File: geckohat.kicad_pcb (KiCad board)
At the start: 2 copper layers, 65 x 56 mm, 37 parts, among them J1 CONN_02X20, J2 TEST_1P, U1 EFM32JG1B100F128GM32, U2 LP2985LV, Y1 38.4 MHz, Y2 32kHz

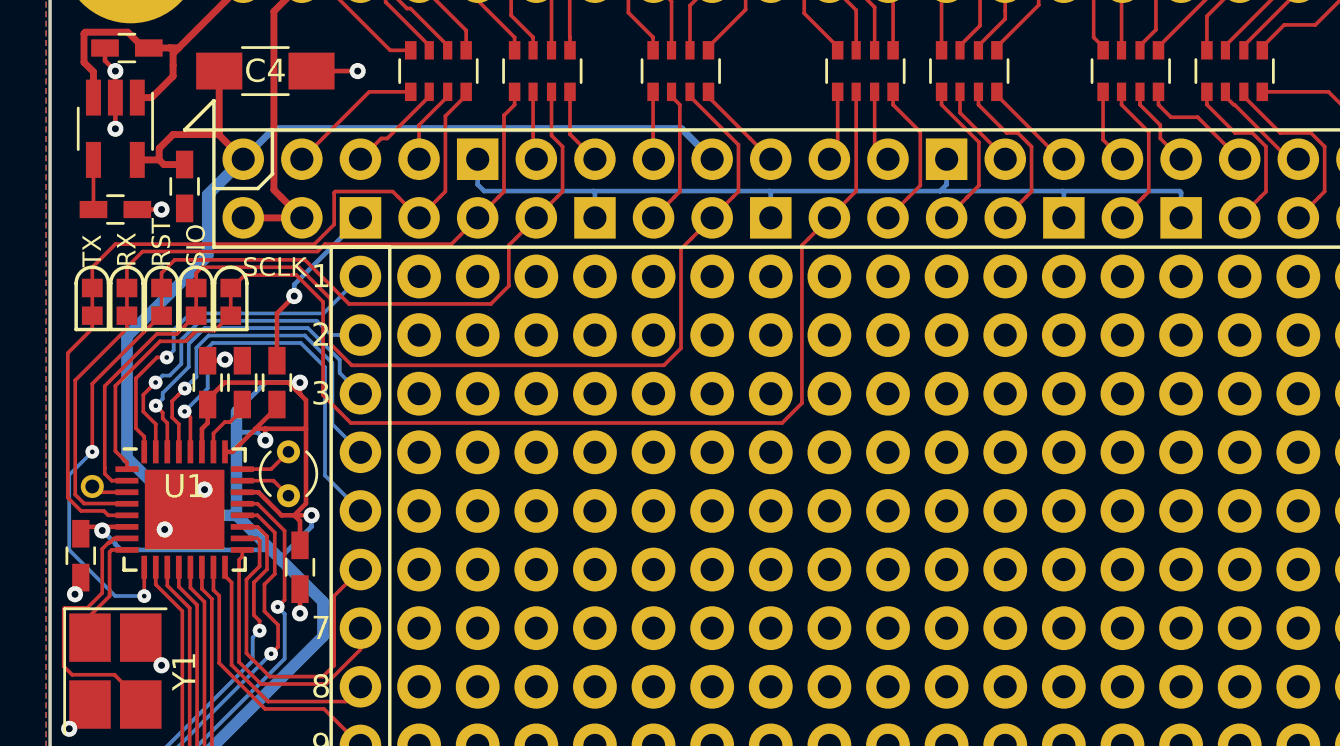
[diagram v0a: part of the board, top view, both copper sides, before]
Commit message: Unknown changes that were lying around
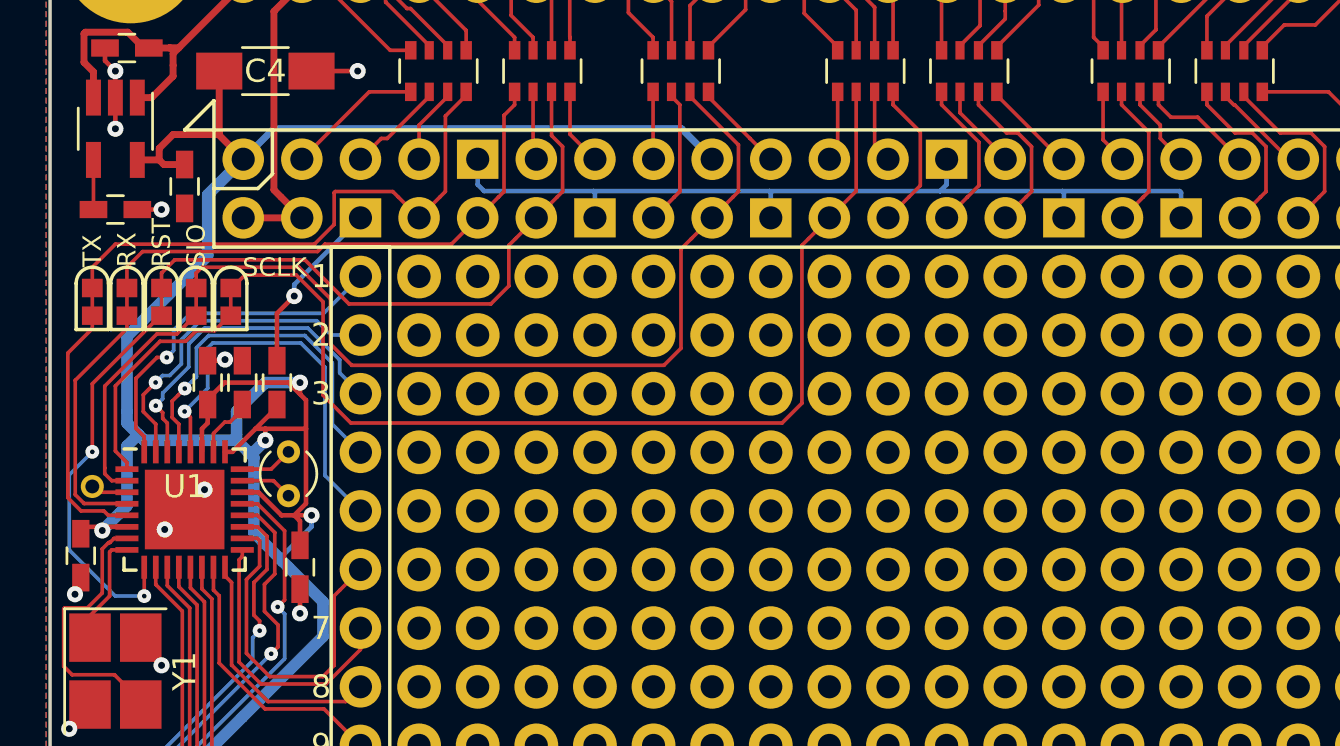
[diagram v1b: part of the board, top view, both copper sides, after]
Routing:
- net VDD: track 139.6 -> 134.2 mm
